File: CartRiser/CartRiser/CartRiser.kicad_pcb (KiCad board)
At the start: 2 copper layers, 46 x 77 mm, 6 parts, among them J1 GROM Port, J2 GROM Port

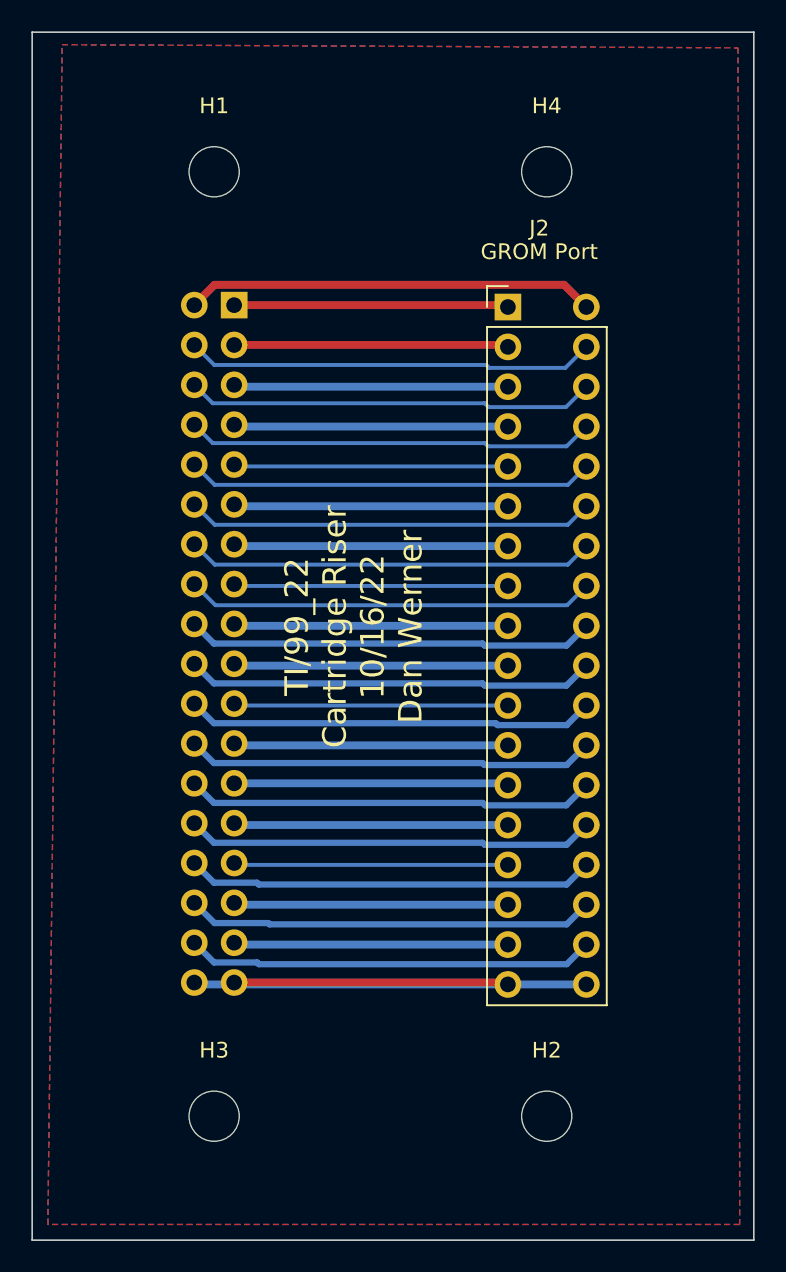
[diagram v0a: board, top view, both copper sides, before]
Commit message: trim cart riser
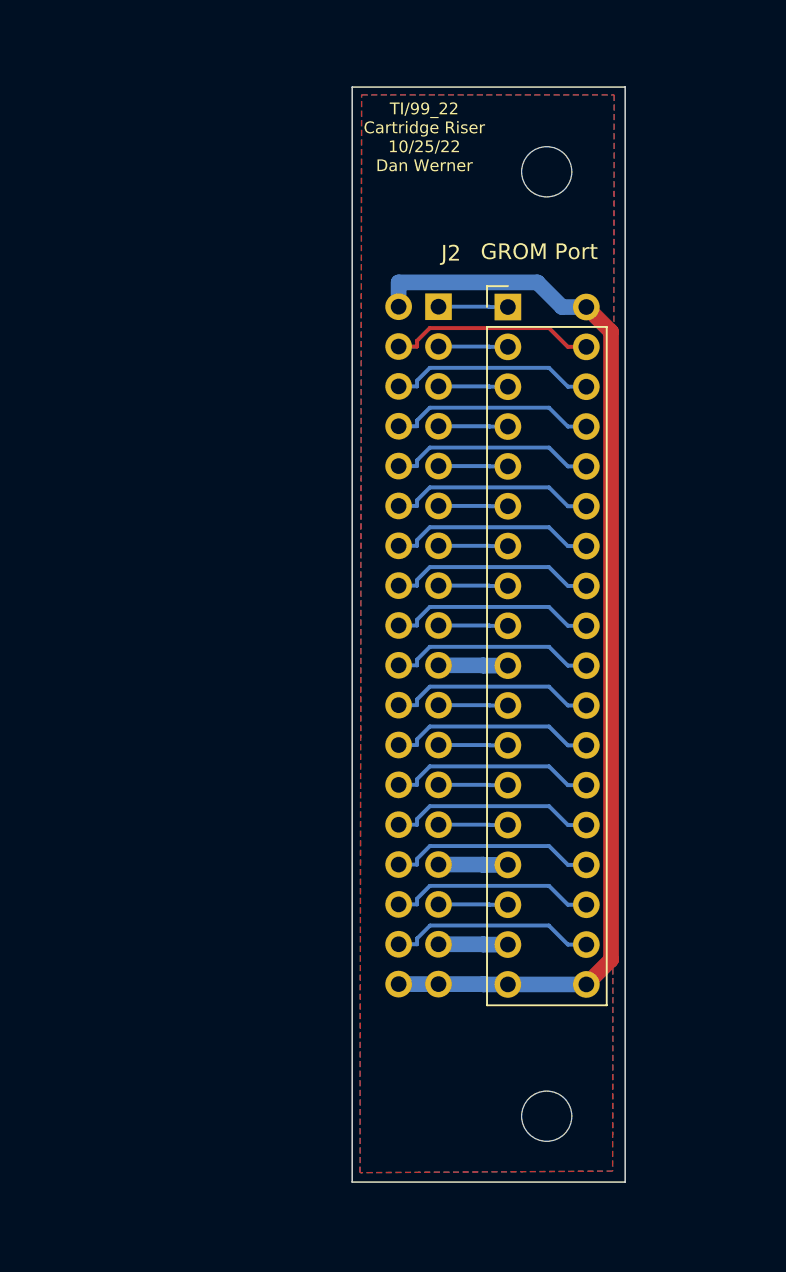
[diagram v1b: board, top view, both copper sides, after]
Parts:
- removed H1, H3: MountingHole, MountingHole:MountingHole_3.2mm_M3
- moved J1 13.0 mm to (166.9, 60.5)
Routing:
- net DBIN: track 17.5 -> 4.43 mm
- net ~{CMRESET}: track 17.5 -> 4.43 mm
- net D7: track 17.5 -> 4.43 mm
- net ~{GS}: track 17.5 -> 4.43 mm
- net D5: track 17.5 -> 4.43 mm
- net D3: track 17.5 -> 4.43 mm
- net -5V: track 17.5 -> 4.43 mm
- net GREADY: track 17.5 -> 4.43 mm
- net D4: track 17.5 -> 4.43 mm
- net D2: track 17.5 -> 4.43 mm
- net D0: track 17.5 -> 4.43 mm
- net VSS: track 17.5 -> 4.43 mm
- net IO_A14: track 17.5 -> 4.43 mm
- net GRMCLK: track 17.5 -> 4.43 mm
- net D6: track 17.5 -> 4.43 mm
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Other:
- board size 46 x 77 mm -> 17.4 x 69.8 mm
- board text added: "TI/99_22 Cartridge Riser 10/25/22 Dan Werner"
- board text removed: "TI/99_22 Cartridge Riser 10/16/22 Dan Werner"
